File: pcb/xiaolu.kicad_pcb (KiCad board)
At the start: 2 copper layers, 51 x 76 mm, 39 parts, among them J1 Conn_01x04_Male, J2 TRRS, SW1 SW_Push, SW10 SW_Push, SW11 SW_Push, SW12 SW_Push, SW13 SW_Push, SW14 SW_Push, SW15 SW_Push, SW16 SW_Push, SW2 SW_Push, SW3 SW_Push, SW4 SW_Push, SW5 SW_Push, SW6 SW_Push, SW7 SW_Push, SW8 SW_Push, SW9 SW_Push, U1 Seeed Studio XIAO SAMD21

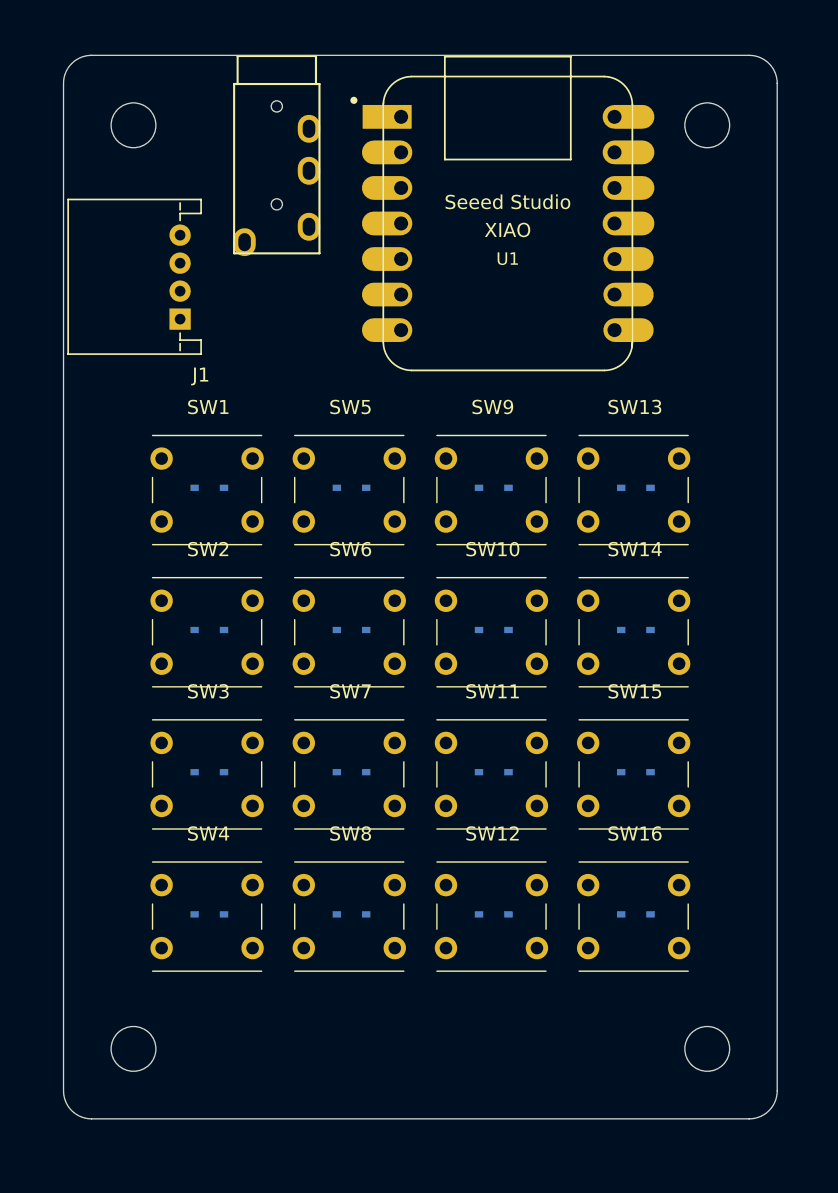
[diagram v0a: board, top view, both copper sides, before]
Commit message: wiring
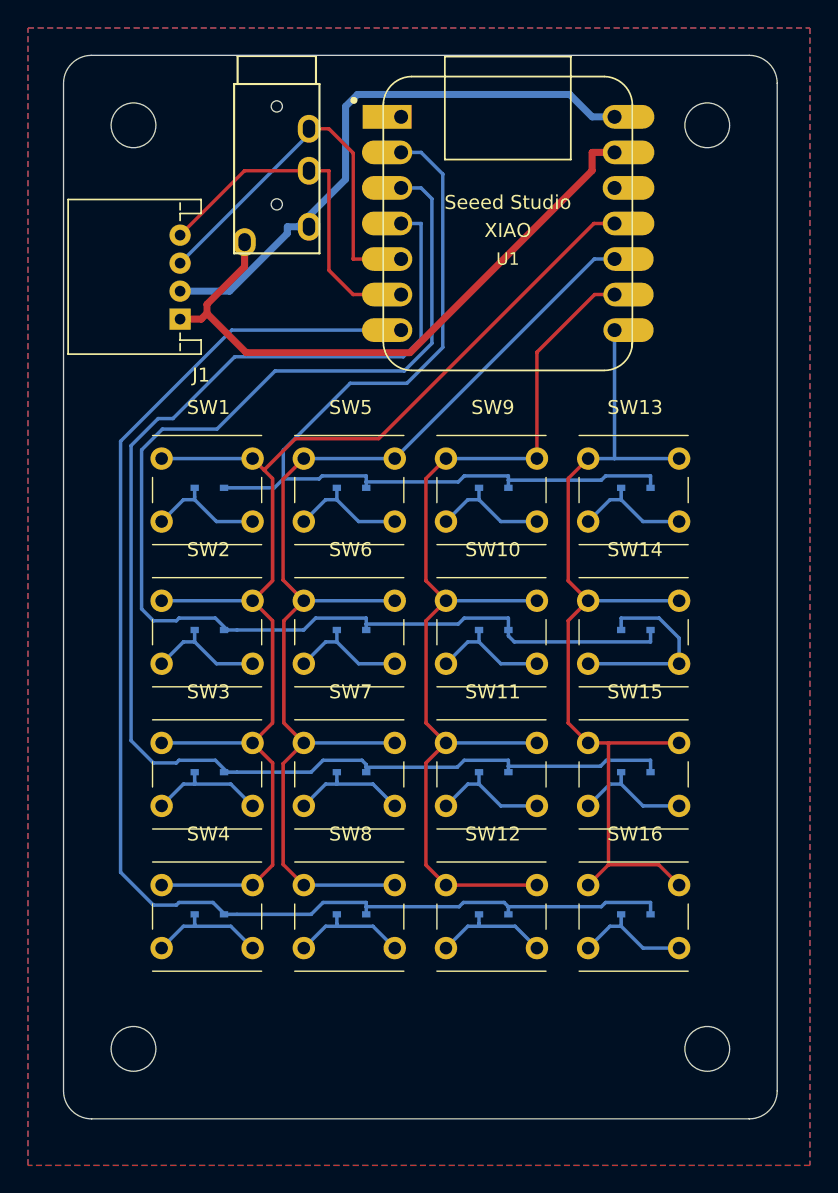
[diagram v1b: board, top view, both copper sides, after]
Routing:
- net row3: track 0.00 -> 96.4 mm
- net row2: track 0.00 -> 96.2 mm
- net col0: track 0.00 -> 92.4 mm
- net row1: track 0.00 -> 89.2 mm
- net col1: track 0.00 -> 81.7 mm
- net col2: track 0.00 -> 74.9 mm
- net col3: track 0.00 -> 67.8 mm
- net row0: track 0.00 -> 66.2 mm
- net GND: track 0.00 -> 45.3 mm
- net +5V: track 0.00 -> 41.6 mm
- net SDA: track 0.00 -> 28.3 mm
- net SCL: track 0.00 -> 25.5 mm
- net Net-(D14-Pad2): track 0.00 -> 13.9 mm
- net Net-(D8-Pad2): track 0.00 -> 8.64 mm
- net Net-(D4-Pad2): track 0.00 -> 8.64 mm
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- added copper zone on B.Cu, net GND
- added copper zone on F.Cu, net GND
